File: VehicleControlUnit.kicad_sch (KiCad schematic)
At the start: 27 parts, among them J10 Precharge_Ready, J11 Precharge+_Conn, J12 Precharge-_Conn, J3 Conn_01x02, J5 MOTOR_CAN_IN, J7 MOTOR_CAN_OUT, J8 CAR_CAN_IN, J9 CAR_CAN_IN, Q1 Q_PMOS_GDS

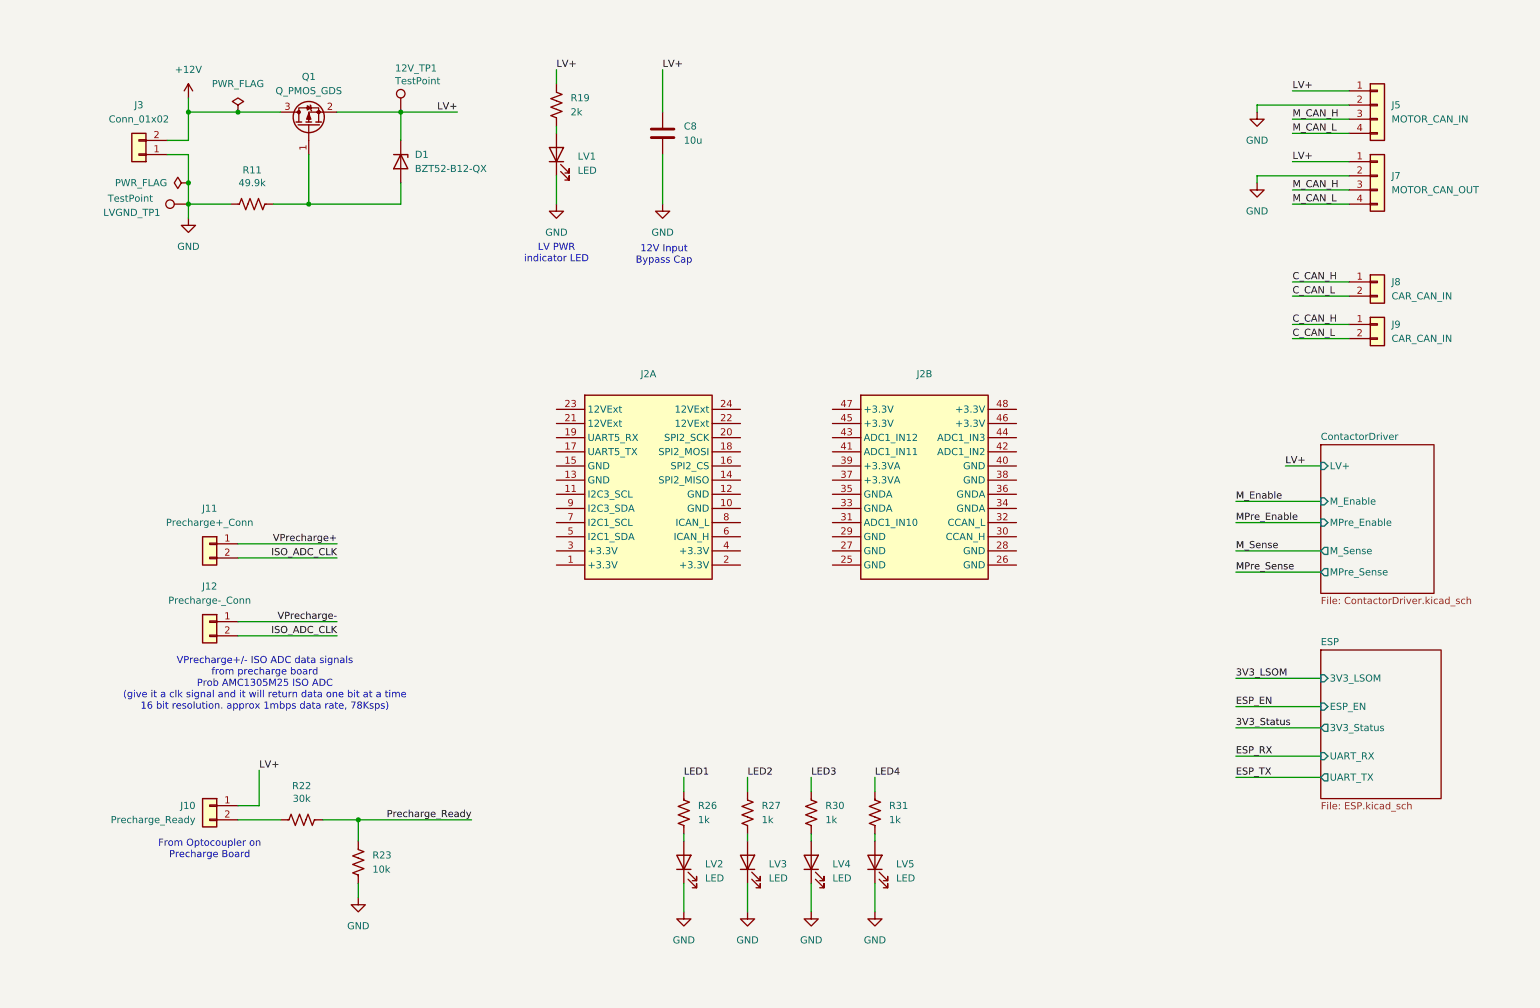
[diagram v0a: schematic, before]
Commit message: pOSPAOBJCO
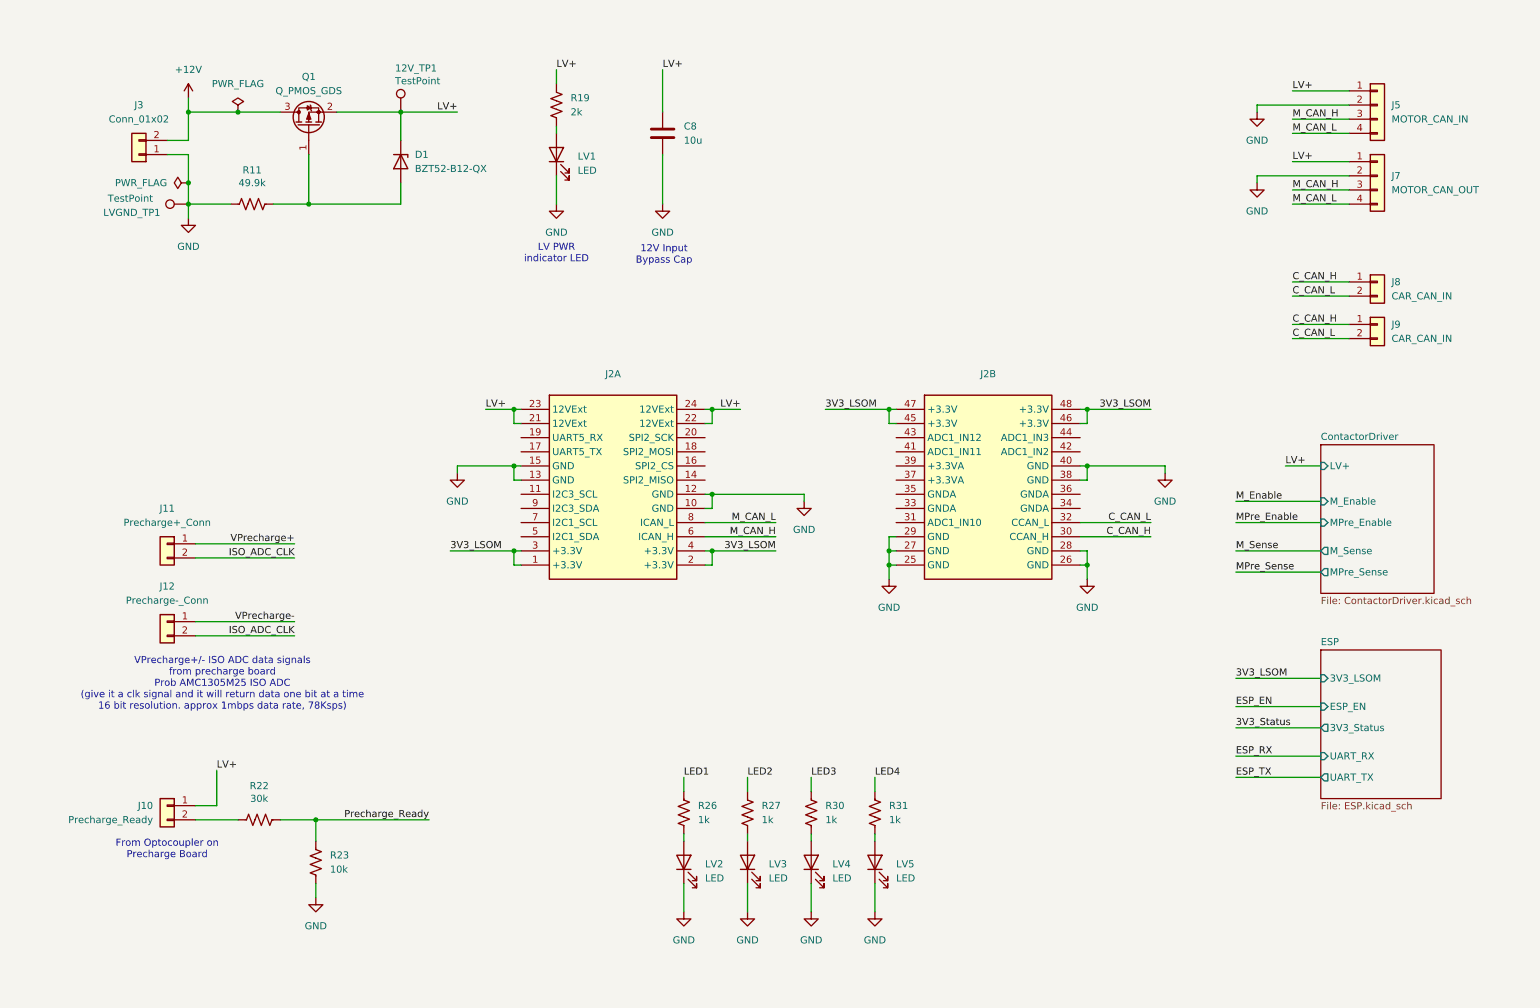
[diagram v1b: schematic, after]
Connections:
- net 3V3_LSOM: now also J2.1 (+3.3V), J2.2 (+3.3V), J2.3 (+3.3V), J2.4 (+3.3V), J2.45 (+3.3V), J2.46 (+3.3V), J2.47 (+3.3V), J2.48 (+3.3V)
- net C_CAN_H: now also J2.30 (CCAN_H)
- net C_CAN_L: now also J2.32 (CCAN_L)
- net GND: now also J2.10 (GND), J2.12 (GND), J2.13 (GND), J2.15 (GND), J2.25 (GND), J2.26 (GND), J2.27 (GND), J2.28 (GND), J2.29 (GND), J2.38 (GND), J2.40 (GND)
- net LV+: now also J2.21 (12VExt), J2.22 (12VExt), J2.23 (12VExt), J2.24 (12VExt)
- net M_CAN_H: now also J2.6 (ICAN_H)
- net M_CAN_L: now also J2.8 (ICAN_L)
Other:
- moved on the sheet: J10, J11, J12, J2A, J2B, R22, R23

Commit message: review LSOM
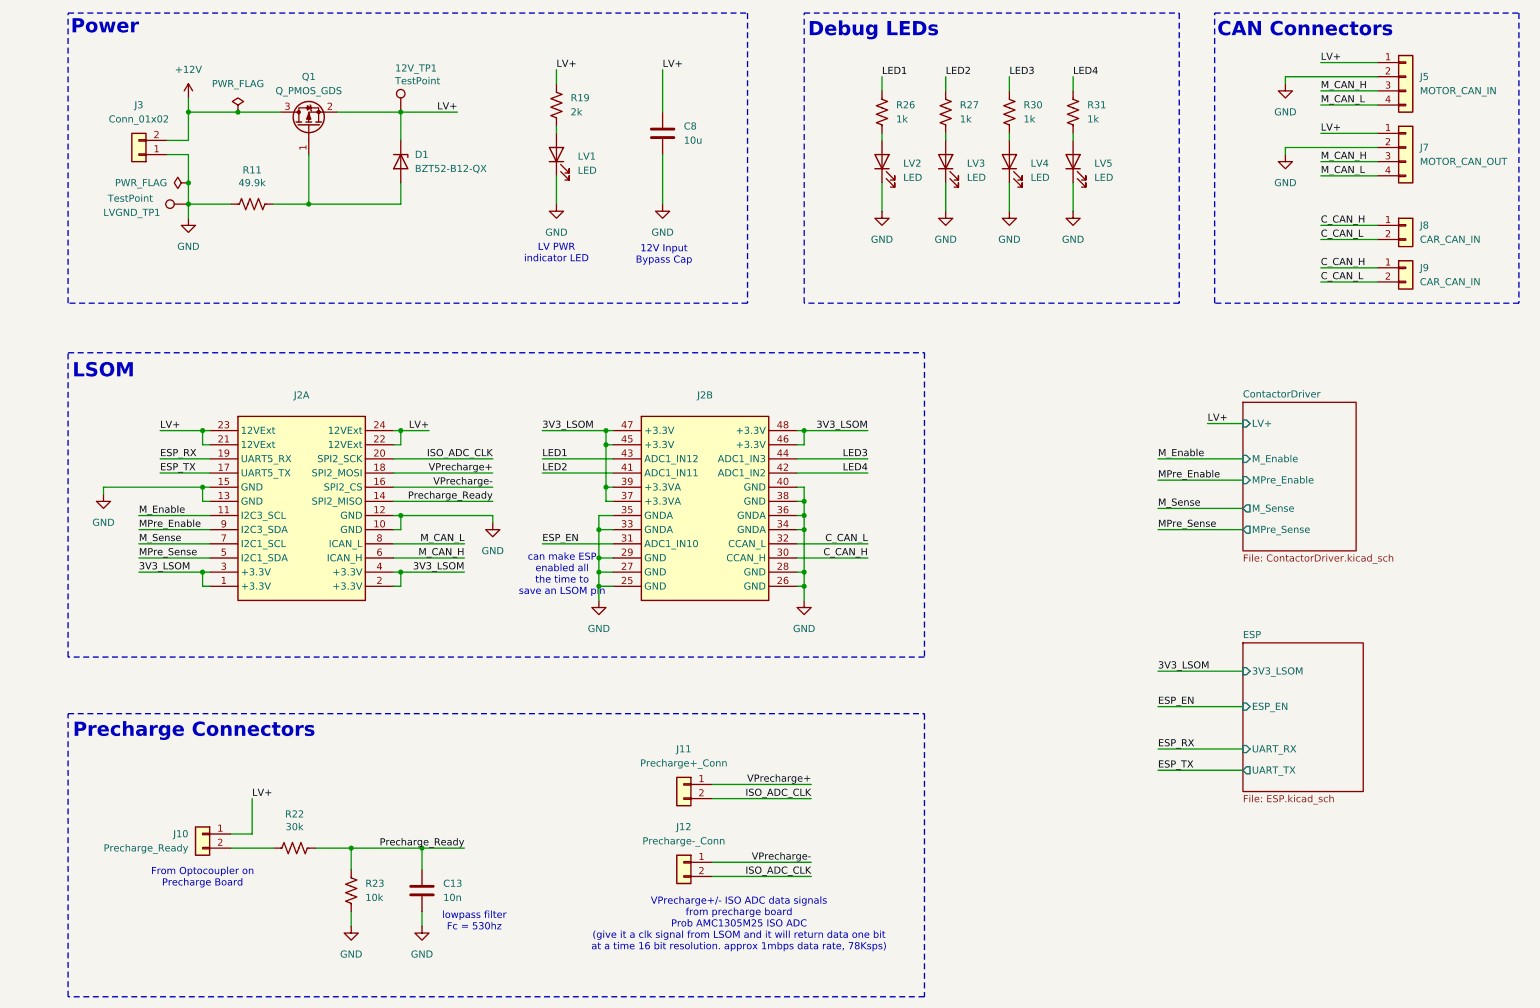
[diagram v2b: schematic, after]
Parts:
- added C13: 10n, Capacitor_SMD:C_0805_2012Metric, symbol Device:C
- J2: footprint (none) -> UTSVT_Special:LeaderSOM
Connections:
- net 3V3_LSOM: now also J2.37 (+3.3VA), J2.39 (+3.3VA)
- net ESP_EN: now also J2.31 (ADC1_IN10)
- net ESP_RX: now also J2.19 (UART5_RX)
- net ESP_TX: now also J2.17 (UART5_TX)
- net GND: now also J2.33 (GNDA), J2.34 (GNDA), J2.35 (GNDA), J2.36 (GNDA), C13.2
- net ISO_ADC_CLK: now also J2.20 (SPI2_SCK)
- net LED1: now also J2.43 (ADC1_IN12)
- net LED2: now also J2.41 (ADC1_IN11)
- net LED3: now also J2.44 (ADC1_IN3)
- net LED4: now also J2.42 (ADC1_IN2)
- net MPre_Enable: now also J2.9 (I2C3_SDA)
- net MPre_Sense: now also J2.5 (I2C1_SDA)
- net M_Enable: now also J2.11 (I2C3_SCL)
- net M_Sense: now also J2.7 (I2C1_SCL)
- net Precharge_Ready: now also J2.14 (SPI2_MISO), C13.1
- net VPrecharge+: now also J2.18 (SPI2_MOSI)
- net VPrecharge-: now also J2.16 (SPI2_CS)
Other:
- sheet ESP ports: added none; removed 3V3_Status
- note added: "CAN Connectors"
- note added: "Debug LEDs"
- note added: "LSOM"
- note added: "Power"
- note added: "Precharge Connectors"
- note added: "VPrecharge+/- ISO ADC data signals from precharge board Prob AMC1305M25 ISO ADC (give it a clk signal from LSOM and it will return data one bit at a time 16 bit resolution. approx 1mbps data rate, 78Ksps)"
- note added: "can make ESP enabled all the time to save an LSOM pin"
- note added: "lowpass filter Fc = 530hz"
- note removed: "VPrecharge+/- ISO ADC data signals from precharge board Prob AMC1305M25 ISO ADC (give it a clk signal and it will return data one bit at a time 16 bit resolution. approx 1mbps data rate, 78Ksps)"
- moved on the sheet: J10, J11, J12, J2A, J2B, J5, J7, J8, J9, LV2, LV3, LV4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
